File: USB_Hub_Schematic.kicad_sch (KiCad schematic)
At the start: 98 parts, among them Q2 BSS84_C114481, Q3 BSS84_C114481, Q4 BSS84_C114481, Q5 BSS84_C114481, U1 USB2517 Chip, U2 USB to microSD, U3 MUX, U4 USB-A F, U5 3.3V CONV, U6 USB-A F, U7 1.8V CONV, U8 TPS2054B, X1 24MHz, X2 24MHz

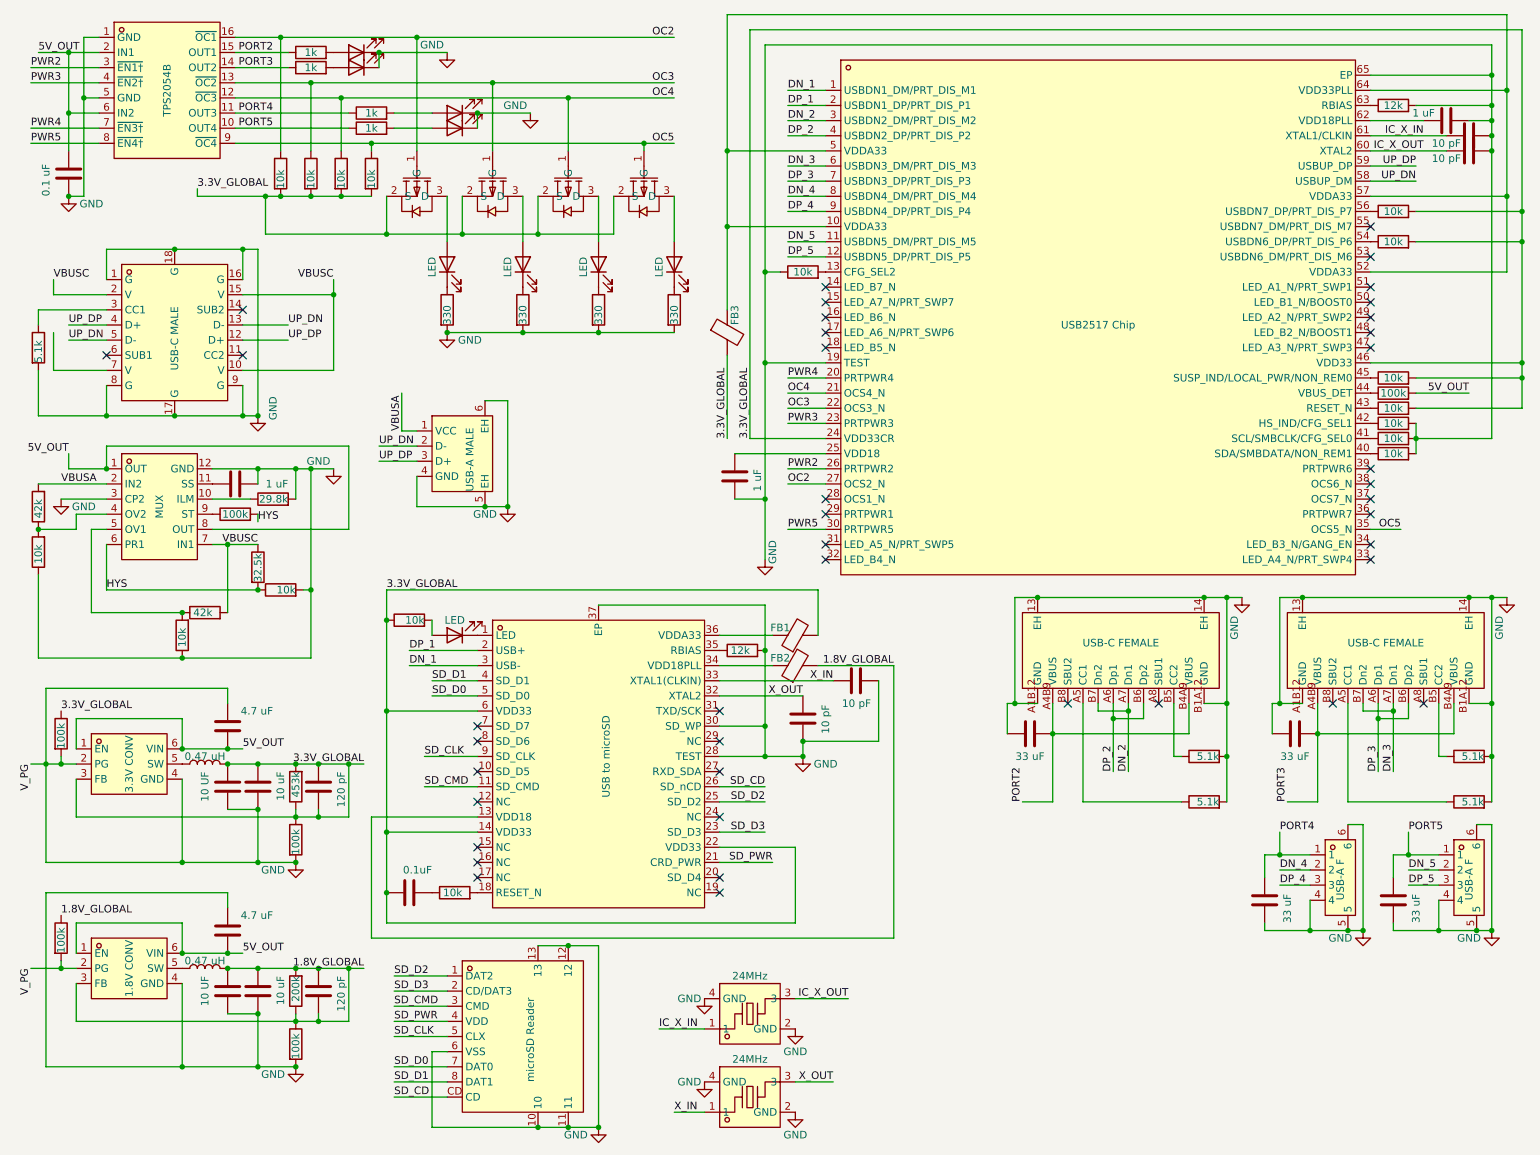
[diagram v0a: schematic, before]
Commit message: Schematic checks
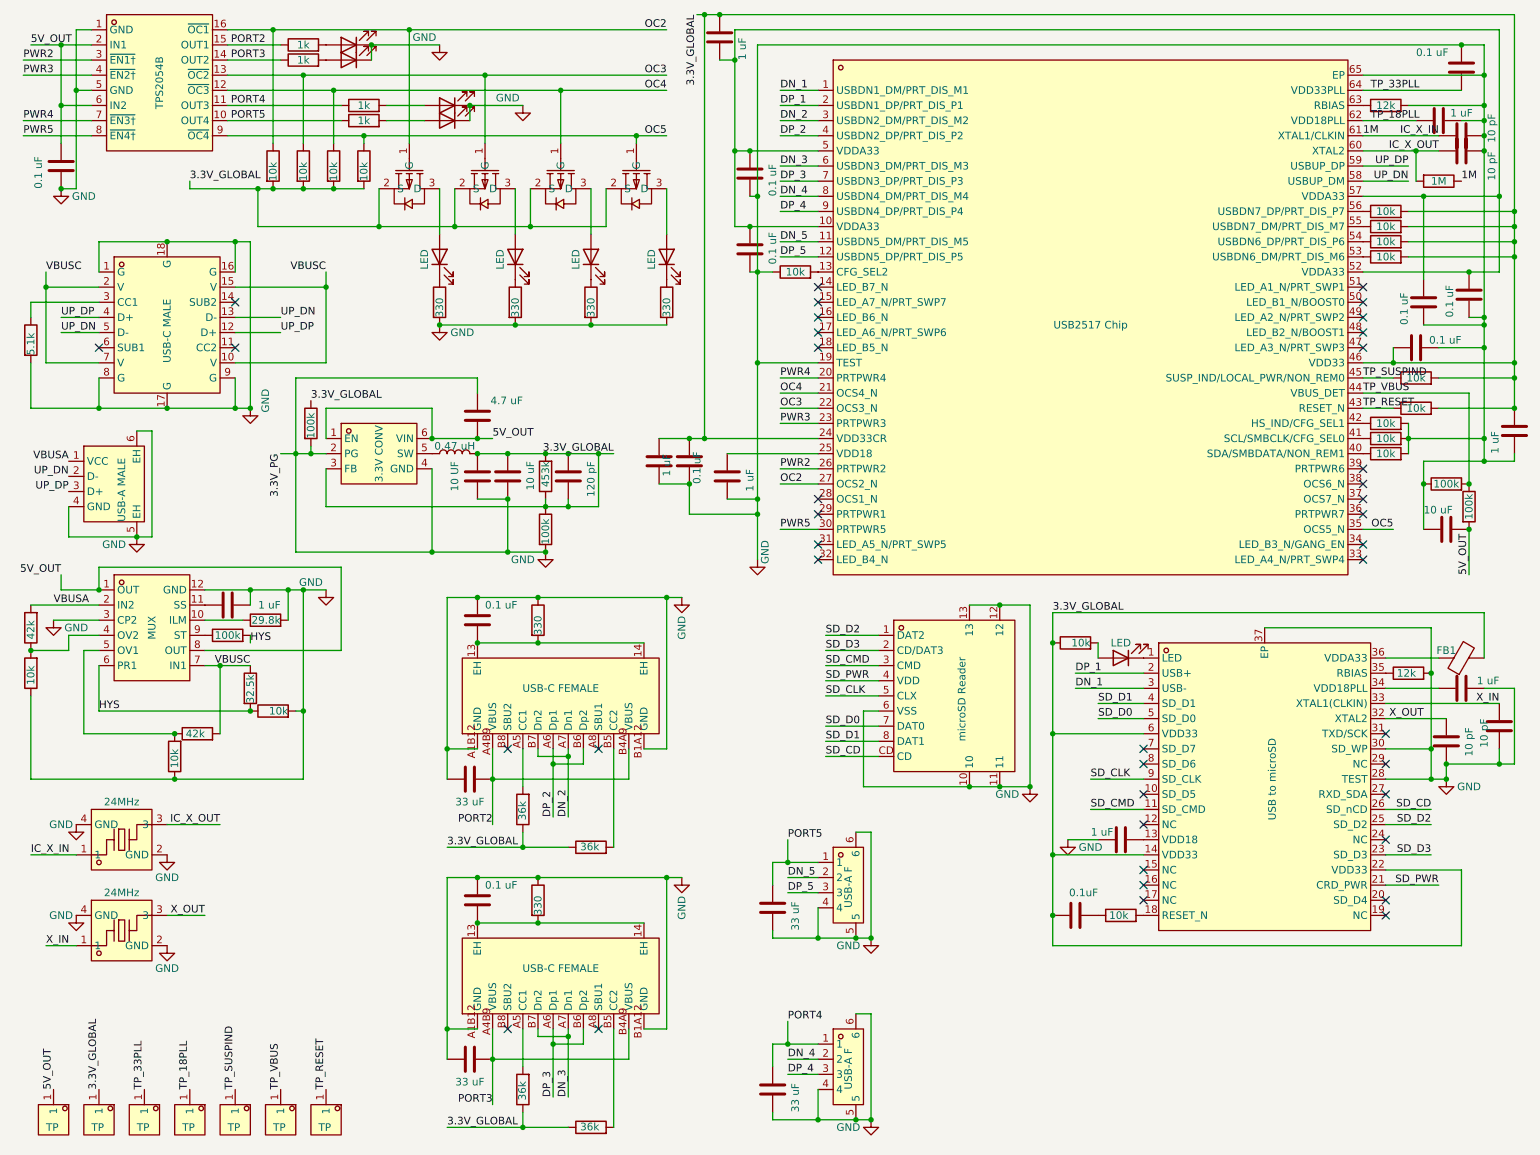
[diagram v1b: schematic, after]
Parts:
- removed C12: 120 pF, symbol Device:C
- removed C17: 33 uF, symbol Device:C
- removed FB2, FB3: FerriteBead, symbol Device:FerriteBead
- removed L2: 0.47 uH, symbol Device:L
- removed R1, R2, R3, R4: 5.1k, Resistor_SMD:R_01005_0402Metric, symbol Device:R
- removed R21: 100k, symbol Device:R
- removed U7: 1.8V CONV, lcsc_easyeda:VSON-6_L1.5-W1.5-P0.50-TL, symbol lcsc_easyeda:TPS62827ADMQR
- removed USB2: USB-C FEMALE, lcsc_easyeda:USB-C-SMD_TYPE-C-16PIN-2MD-073, symbol lcsc_easyeda:TYPE-C16PIN2MD
- added C23, C24, C25, C29, C32, C36: 0.1 uF, symbol Device:C
- added C26, C27, C30, C31, C35: 1 uF, symbol Device:C
- added C28: 10 uF, symbol Device:C
- added C34: 33 uF, symbol Device:C
- added R34, R47: 100k, symbol Device:R
- added R46: 10k, symbol Device:R
- added R48: 1M, symbol Device:R
- added R49, R50, R52: 36k, Resistor_SMD:R_01005_0402Metric, symbol Device:R
- added R51: 330, symbol Device:R
- added U10, U11, U12, U13, U14, U15, U9: TP, lcsc_easyeda:TEST-SMD_L2.7-W1.0, symbol lcsc_easyeda:5015
- added USB5: USB-C FEMALE, lcsc_easyeda:USB-C-SMD_TYPE-C-16PIN-2MD-073, symbol lcsc_easyeda:TYPE-C16PIN2MD
- C10: value 10 UF -> 0.1 uF
- C11: value 10 uF -> 0.1 uF
- C9: value 4.7 uF -> 0.1 uF
- R22: value 200k -> 330
- R23: value 100k -> 36k; footprint (none) -> Resistor_SMD:R_01005_0402Metric
- R26: value 100k -> 10k
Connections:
- net 3.3V_GLOBAL: now also R23.1, R26.2, C30.1, C31.1, C32.1, C35.1, C36.1, R46.2, R49.1, R50.1, R52.1, U10.1
- net 5V_OUT: now also C28.1, R34.2, U9.1; no longer C9.1, R26.2
- net DN_3: now also USB5.A7 (Dn1), USB5.B7 (Dn2)
- net DP_3: now also USB5.A6 (Dp1), USB5.B6 (Dp2)
- net GND: now also C3.1, R22.1, C23.2, C24.1, C25.2, C26.2, C27.1, C28.2, C29.2, C30.2, C32.2, C34.1, C35.2, C36.2, R47.1, R51.1, USB5.A1B12 (GND), USB5.B1A12 (GND); no longer C3.2, R23.2, USB1.13 (EH), USB1.14 (EH)
- net IC_X_OUT: now also R48.2
- net PORT3: now also C34.2, USB5.A4B9 (VBUS), USB5.B4A9 (VBUS)
- net VBUSC: now also USB4.7 (V)
- net X_IN: now also C3.2; no longer C3.1
- net TP_SUSPIND: now reaches R37.1, U1.45 (SUSP_IND/LOCAL_PWR/NON_REM0)
- net TP_SUSPIND: now also U13.1
- net at U1.10 (VDDA33), U1.5 (VDDA33), U1.52 (VDDA33)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: now also C9.1, C23.1, C25.1, C29.1, C31.2; no longer U1.64 (VDD33PLL)
- net at U2.34 (VDD18PLL): now also C26.1
- net at USB1.A5 (CC1): now also R49.2
- net TP_RESET: now reaches R41.1, U1.43 (RESET_N)
- net TP_RESET: now also U15.1
- net at R26.1: now also U1.55 (USBDN7_DM/PRT_DIS_M7); no longer U1.44 (VBUS_DET)
- net at U1.53 (USBDN6_DM/PRT_DIS_M6): now also R46.1
- net TP_18PLL: now reaches C22.1, U1.62 (VDD18PLL)
- net TP_18PLL: now also U12.1
- net at USB1.B5 (CC2): now also R23.2
- removed net 1.8V_GLOBAL: C10.2, C11.2, R22.1, R22.2, R23.1, U2.13 (VDD18)
- net IC_X_IN renamed 1M
- net 1M: now also R48.1
- new net: R50.2, USB5.A5 (CC1)
- new net: C11.2, R51.2, USB5.13 (EH), USB5.14 (EH)
- new net: C27.2, U2.13 (VDD18)
- new net: C10.2, R22.2, USB1.13 (EH), USB1.14 (EH)
- new net: R52.2, USB5.B5 (CC2)
- new net TP_33PLL: C24.2, U1.64 (VDD33PLL), U11.1
- new net TP_VBUS: R34.1, R47.2, U1.44 (VBUS_DET), U14.1
- no-connect marks 42 -> 40
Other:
- moved on the sheet: FB1
